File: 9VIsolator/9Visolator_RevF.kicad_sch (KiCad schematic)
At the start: 15 parts, among them J1 IN, J2 OUT, U1 B0912S-1WR3, U2 LD1117AG-AD-AB3-A

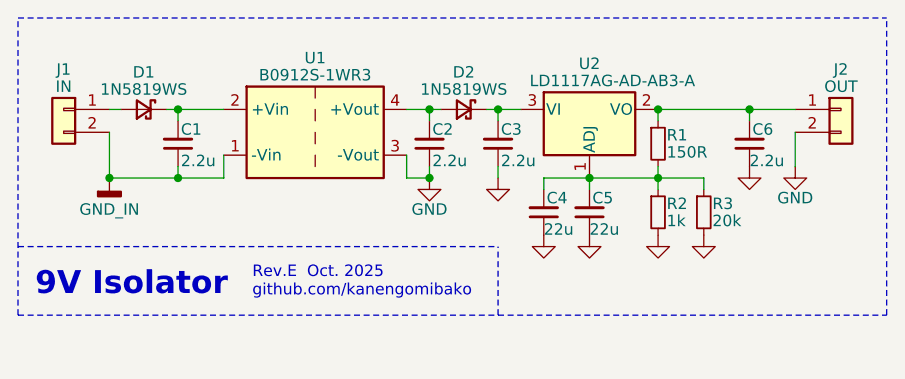
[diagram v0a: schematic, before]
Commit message: Update KiCad data
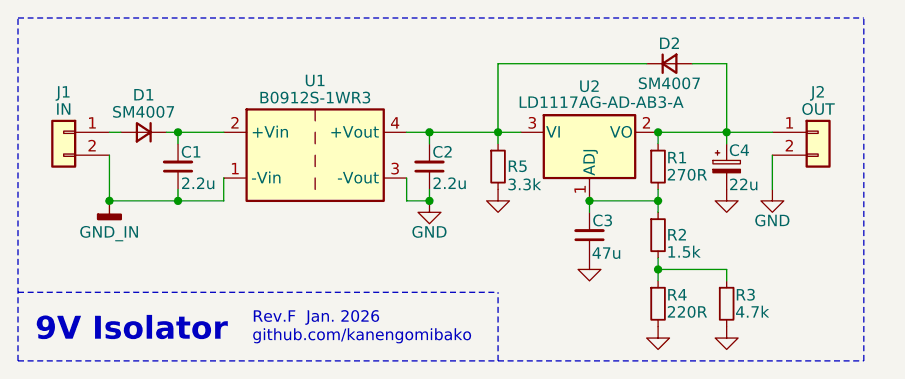
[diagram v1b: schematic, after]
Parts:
- removed C4, C5: 22u, Capacitor_SMD:C_0805_2012Metric, symbol Device:C_Small
- removed C6: 2.2u, Capacitor_SMD:C_0805_2012Metric, symbol Device:C_Small
- removed D2: 1N5819WS, myFoot:my_D_SOD-323, symbol Device:D_Schottky_Small
- added C4: 22u, Capacitor_Tantalum_SMD:CP_EIA-3528-15_AVX-H, symbol Device:C_Polarized_Small
- added D2: SM4007, Diode_SMD:D_SOD-123F, symbol Device:D_Small
- added R3: 4.7k, Resistor_SMD:R_0603_1608Metric, symbol Device:R_Small
- added R5: 3.3k, Resistor_SMD:R_0603_1608Metric, symbol Device:R_Small
- C1, C2: LCSC (none) -> C377773; MPN C377773 -> (none)
- C3: value 2.2u -> 47u; footprint Capacitor_SMD:C_0805_2012Metric -> Capacitor_SMD:C_1206_3216Metric; LCSC (none) -> C96123; MPN C377773 -> (none)
- D1: value 1N5819WS -> SM4007; footprint myFoot:my_D_SOD-323 -> Diode_SMD:D_SOD-123F; symbol Device:D_Schottky_Small -> Device:D_Small; LCSC (none) -> C64898; MPN C191023 -> (none)
- J1, J2: now left out of the parts list
- R1: value 150R -> 270R; LCSC (none) -> C22966; MPN C22808 -> (none)
- R2: value 1k -> 1.5k; footprint Resistor_SMD:R_0805_2012Metric -> Resistor_SMD:R_0603_1608Metric; LCSC (none) -> C22843; MPN C17513 -> (none)
- R4: renamed from R3; value 20k -> 220R; LCSC (none) -> C22962; MPN C4184 -> (none)
- U1: MPN C19272674 -> (none); now left out of the parts list
- U2: footprint myFoot:SOT-89-3-rotate -> Package_TO_SOT_SMD:SOT-89-3; LCSC (none) -> C80540; MPN C80540 -> (none)
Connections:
- net GND: now also C4.2, R3.2, R5.2; no longer R2.2
- net at C2.2, U1.4 (+Vout): now also U2.3 (VI), D2.1 (K), R5.1
- net at R1.2, R2.1, U2.1 (ADJ): now also C3.2; no longer R4.1
- net at J2.1 (Pin_1), R1.1, U2.2 (VO): now also C4.1, D2.2 (A)
- new net: R2.2, R3.1, R4.1
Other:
- note added: "Rev.F Jan. 2026 github.com/kanengomibako"
- note removed: "Rev.E Oct. 2025 github.com/kanengomibako"
- moved on the sheet: C1, C2, D1, J1, J2, R1, R4, U1, U2
